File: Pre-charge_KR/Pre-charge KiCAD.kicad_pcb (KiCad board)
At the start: 2 copper layers, 62.9 x 86.1 mm, 60 parts, among them IC1 AL5890-10D-13, IC2 TLV1701AIDBVT, J1 Conn_01x02, J2 Conn_01x06, J3 Conn_01x02, J4 Conn_01x02, K2 G5Q-1A4-DC12, K3 67-1-A-12/2D, Q1 2N7000, Q2 2N7000, Q4 2N7000, U1 HCPL-817-000E, U10 LM7805MPX/NOPB, U13 HCPL-817-000E, U2 LM339N/NOPB, U3 SN74AHCT1G08DBVR, U7 LM741CN/NOPB, U8 SN74AHC1G04DBVRE4

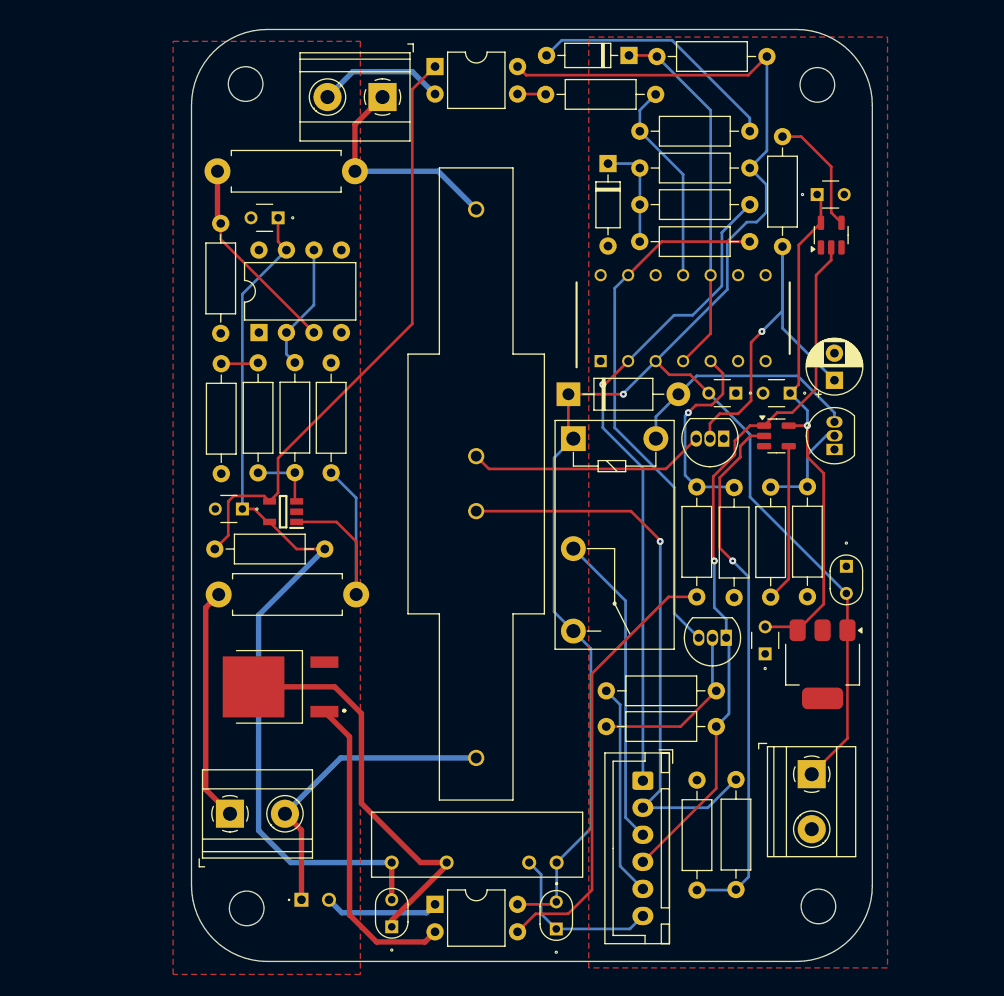
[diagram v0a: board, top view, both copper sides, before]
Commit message: precharge complete
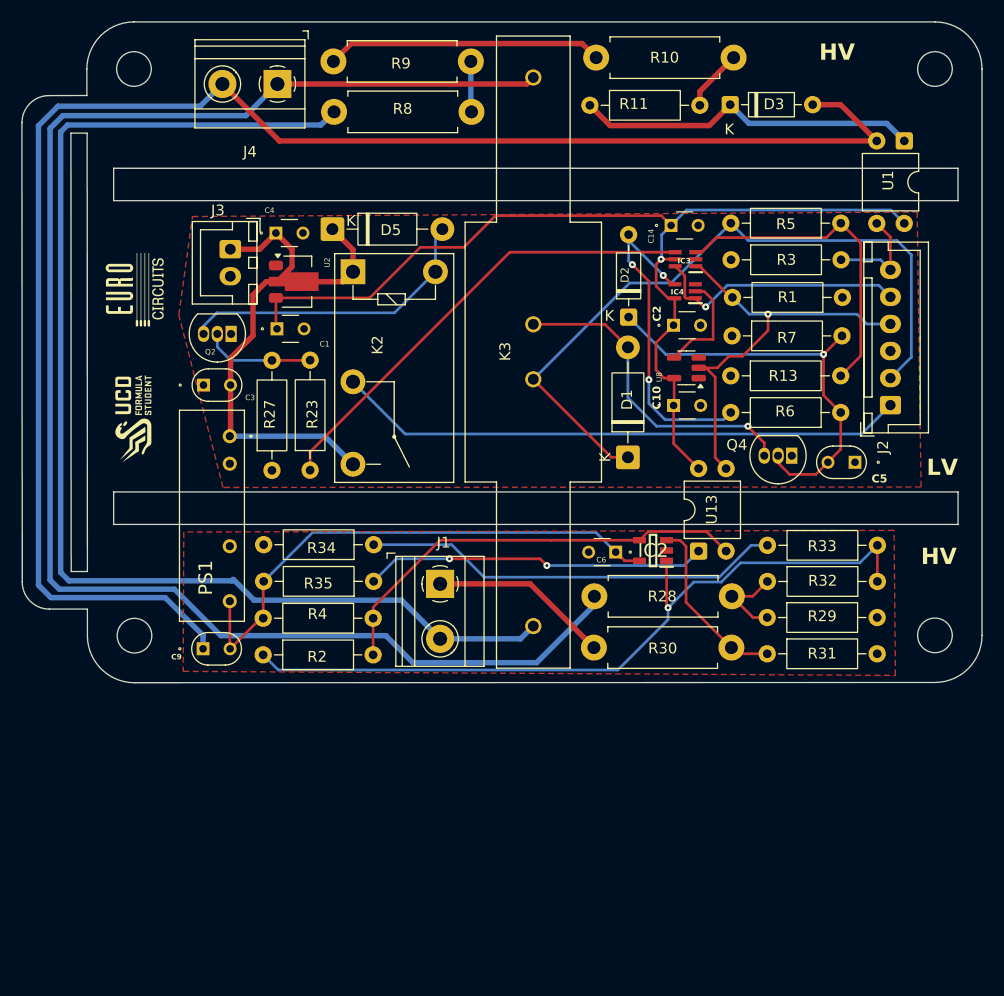
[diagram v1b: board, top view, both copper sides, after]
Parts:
- removed C11: 0.1uF, FA14_Capacitor:FA18X7R1H104KNU00
- removed C7: 0.22uF, FA14_Capacitor:FA14X7R1H224KNU00
- removed IC1: AL5890-10D-13, AL589010D13:AL589010D13
- removed LED1: LTL-1CHG, LTL1CHG:LTL1CHG
- removed Q1: 2N7000, Package_TO_SOT_THT:TO-92_Inline
- removed R12: 20k, Resistor_THT:R_Axial_DIN0207_L6.3mm_D2.5mm_P10.16mm_Horizontal
- removed R24: 1M, Resistor_THT:R_Axial_DIN0207_L6.3mm_D2.5mm_P10.16mm_Horizontal
- removed R36: 6.8k, Resistor_THT:R_Axial_DIN0207_L6.3mm_D2.5mm_P10.16mm_Horizontal
- removed R37: 4.7k, Resistor_THT:R_Axial_DIN0207_L6.3mm_D2.5mm_P10.16mm_Horizontal
- removed the REF** at (97.4, 35.8)
- removed the REF** at (44.7, 111.9)
- removed the REF** at (97.5, 111.7)
- removed the REF** at (44.6, 35.7)
- removed U10: LM7805MPX/NOPB, Package_TO_SOT_SMD:SOT-223-3_TabPin2
- removed U3: SN74AHCT1G08DBVR, Package_TO_SOT_SMD:SOT-23-5
- removed U7: LM741CN/NOPB, Package_DIP:DIP-8_W7.62mm
- added C5: 2.2uF, FA14_Capacitor:FA14X7R1H224KNU00, F.Cu at (100.9, 70.7)
- added D2: 1N4148, Diode_THT:D_DO-35_SOD27_P7.62mm_Horizontal, F.Cu at (79.9, 57.3)
- added IC3: SN74LVC1G11DCKRE4, SOT65:SOT65P210X110-6N, F.Cu at (85.2, 51.9)
- added IC4: SN74LVC1G08IDCKRQ1, AND:SOT65P210X110-5N, F.Cu at (85.2, 54.9)
- added R10: 56k, Resistor_THT:R_Axial_DIN0411_L9.9mm_D3.6mm_P12.70mm_Horizontal, F.Cu at (76.9, 33.3)
- added R3: 100k, Resistor_THT:R_Axial_DIN0207_L6.3mm_D2.5mm_P10.16mm_Horizontal, F.Cu at (89.4, 52.0)
- added R6: 100k, Resistor_THT:R_Axial_DIN0207_L6.3mm_D2.5mm_P10.16mm_Horizontal, F.Cu at (99.5, 66.1)
- added REF**: MountingHole_3.2mm_M3, MountingHole:MountingHole_3.2mm_M3, F.Cu at (108.2, 86.7)
- added REF**: MountingHole_3.2mm_M3, MountingHole:MountingHole_3.2mm_M3, F.Cu at (108.2, 34.3)
- added REF**: MountingHole_3.2mm_M3, MountingHole:MountingHole_3.2mm_M3, F.Cu at (34.3, 86.7)
- added REF**: MountingHole_3.2mm_M3, MountingHole:MountingHole_3.2mm_M3, F.Cu at (34.2, 34.3)
- C1, C4: value 0.1uF -> 1uF
- C2: value 10uF -> 0.1uF; footprint Capacitor_THT:CP_Radial_D5.0mm_P2.50mm -> FA14_Capacitor:FA18X7R1H104KNU00
- D1: value TZX3V9C-TAP -> 1N4001; footprint Diode_THT:D_DO-35_SOD27_P7.62mm_Horizontal -> Diode_THT:D_DO-41_SOD81_P10.16mm_Horizontal
- D3: value TZX3V0B-TR -> 1N4148
- J3: footprint Phoenix 1x2 Connector:Phoenix_1x2_1729128 -> Connector_JST:JST_XH_B2B-XH-A_1x02_P2.50mm_Vertical
- R1: value 1.5k -> 100k
- R11: value 10k -> 330
- R2: value 1.5k -> 1M
- R32, R33, R7: value 10k -> 100k
- R34: value 180k -> 1.8M
- R35: value 1k -> 2.2k
- R4: value 6.8k -> 10k
- R5: value 4.7k -> 27k
- R8: value 10k -> 56k; footprint Resistor_THT:R_Axial_DIN0207_L6.3mm_D2.5mm_P10.16mm_Horizontal -> Resistor_THT:R_Axial_DIN0411_L9.9mm_D3.6mm_P12.70mm_Horizontal
- R9: value 100 -> 56k; footprint Resistor_THT:R_Axial_DIN0207_L6.3mm_D2.5mm_P10.16mm_Horizontal -> Resistor_THT:R_Axial_DIN0411_L9.9mm_D3.6mm_P12.70mm_Horizontal
- U2: value LM339N/NOPB -> MCP1703AT-3302E/MBVAO; footprint LM339N:DIP794W53P254L1930H508Q14N -> Package_TO_SOT_SMD:SOT-89-3
- U8: value SN74AHC1G04DBVRE4 -> SN74LVC1G04QDBVRQ1
- moved U1 82.8 mm to (105.4, 41.0), turned to -90 degrees
- moved J3 72.4 mm to (43.1, 51.0)
- moved R2 72.3 mm to (46.2, 88.5), turned to 0 degrees
- moved R9 62.4 mm to (65.4, 33.6)
- moved R29 62.2 mm to (92.8, 85.0), turned to 0 degrees
- moved C3 59.9 mm to (40.7, 63.5), turned to 0 degrees
- moved R33 57.6 mm to (102.9, 78.3), turned to 180 degrees
- moved R11 57.4 mm to (76.4, 37.7)
- moved Q2 56.8 mm to (43.2, 58.8), turned to 180 degrees
- moved U13 51.0 mm to (86.4, 78.9), turned to 90 degrees
- moved R27 50.8 mm to (47.0, 71.4)
- moved PS1 49.6 mm to (43.1, 68.3), turned to -90 degrees
- moved R32 48.1 mm to (92.8, 81.7), turned to 0 degrees
- moved R28 45.1 mm to (76.8, 83.1), turned to 0 degrees
- moved C4 45.0 mm to (47.4, 49.5), turned to 0 degrees
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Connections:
- C1 pad 1: 12V_HV -> 3.3V
- C1 pad 2: TS- -> GLV-
- C10 pad 1: 5V -> 3.3V
- C14 pad 1: 5V -> 3.3V
- C2 pad 1: Precharge NOT done -> 3.3V
- C4 pad 1: GLV- -> GLV+
- C4 pad 2: GLV+ -> GLV-
- D1 pad 1: 3V9 -> SDWN_PC
- D1 pad 2: GLV- -> Net-(D1-A)
- D3 pad 1: 3Vref -> Net-(D3-K)
- D3 pad 2: GLV- -> TS-
- J2 pad 1: Precharge_ON -> Shutdown_AIR1+
- J2 pad 3: Shutdown_AIR1+ -> GLV-
- J2 pad 4: Precharge_done/Close_AIR1 -> Precharge_done
- J2 pad 5: TS_activate -> Precharge_EN
- J2 pad 6: GLV- -> Precharge_ON
- K3 pad 3: Net-(Q4-D) -> Net-(D1-A)
- Q4 pad 2: Precharge NOT done -> Net-(D2-K)
- Q4 pad 3: Net-(Q4-D) -> Net-(D1-A)
- R1 pad 1: GLV+ -> GLV-
- R1 pad 2: 3V9 -> Precharge_done
- R11 pad 1: Net-(Q1-G) -> Net-(D3-K)
- R11 pad 2: Precharge_done/Close_AIR1 -> Net-(R10-Pad2)
- R13 pad 2: Net-(R12-Pad1) -> Net-(IC3-B)
- R2 pad 1: GLV+ -> Net-(IC2-IN+)
- R2 pad 2: 3Vref -> Net-(IC2-OUT)
- R28 pad 2: Net-(U7-+) -> Net-(R28-Pad2)
- R29 pad 1: Net-(U7-+) -> Net-(R28-Pad2)
- R30 pad 2: Net-(IC2-IN+) -> Net-(IC2-IN-)
- R31 pad 1: Net-(IC2-IN+) -> Net-(IC2-IN-)
- R32 pad 1: Net-(U7--) -> Net-(R28-Pad2)
- R32 pad 2: Net-(IC2-IN-) -> Net-(IC2-IN+)
- R33 pad 1: Net-(IC2-IN-) -> Net-(IC2-IN+)
- R35 pad 1: Net-(IC2-OUT) -> Net-(R35-Pad1)
- R4 pad 1: Net-(R4-Pad1) -> Net-(IC2-OUT)
- R4 pad 2: Net-(U2A-+) -> 12V_HV
- R5 pad 1: Net-(U2A-+) -> Net-(IC3-B)
- R5 pad 2: GLV- -> SDWN_PC
- R7 pad 1: Precharge_ON -> GLV-
- R7 pad 2: 3V9 -> Net-(D2-K)
- R8 pad 1: Net-(Q1-D) -> PRE_RESIST+
- R8 pad 2: 3V9 -> Net-(R8-Pad2)
- R9 pad 1: Net-(Q1-G) -> Net-(R8-Pad2)
- R9 pad 2: TS_activate -> Net-(R10-Pad1)
- U1 pad 1: Net-(LED1-K) -> Net-(D3-K)
- U1 pad 2: Net-(IC1-IN) -> TS-
- U1 pad 3: Net-(R4-Pad1) -> Precharge_ON
- U1 pad 4: GLV+ -> 3.3V
- U13 pad 1: Net-(IC2-OUT) -> Net-(R35-Pad1)
- U13 pad 2: TS- -> Net-(IC2-OUT)
- U13 pad 3: Net-(R36-Pad2) -> Precharge_done
- U13 pad 4: GLV+ -> 3.3V
- U2 pad 2: Precharge_ON -> GLV+
- U2 pad 3: GLV+ -> 3.3V
- U8 pad 2: Precharge_done/Close_AIR1 -> Precharge_done
- U8 pad 4: Net-(R24-Pad1) -> Precharge NOT done
- U8 pad 5: 5V -> 3.3V
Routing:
- net TS+: track 20.6 -> 144.8 mm
- net GLV+: track 170.2 -> 52.0 mm, vias 1 -> 0
- net TS-: track 49.2 -> 149.3 mm
- net 3.3V: track 0.00 -> 93.9 mm, vias 0 -> 1
- net PRE_RESIST+: track 28.4 -> 113.5 mm
- net Precharge_done/Close_AIR1: track 66.8 -> 0.00 mm, vias 1 -> 0
- net Precharge_ON: track 61.5 -> 9.76 mm, vias 1 -> 0
- net Net-(Q1-D): track 49.8 -> 0.00 mm
- net Net-(R12-Pad1): track 49.6 -> 0.00 mm, vias 1 -> 0
- net 5V: track 49.2 -> 0.00 mm, vias 1 -> 0
- net Net-(IC2-IN+): track 23.3 -> 70.5 mm, vias 0 -> 1
- net Net-(R4-Pad1): track 41.1 -> 0.00 mm
- net Precharge_done: track 0.00 -> 40.3 mm, vias 0 -> 1
- net GLV-: track 39.5 -> 0.00 mm
- net Net-(D2-K): track 0.00 -> 39.1 mm, vias 0 -> 1
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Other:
- board size 62.9 x 86.1 mm -> 88.7 x 61.1 mm
- board text added: "HV"
- board text added: "LV"
